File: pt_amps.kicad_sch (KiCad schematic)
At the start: 39 parts, among them J25 Conn_01x04_Female, U11 LM324DT

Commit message: not sure if anything has changed but this is the last commit before moving to two LCs
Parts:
- J25: footprint Connector_PinHeader_2.54mm:PinHeader_1x04_P2.54mm_Vertical -> Connector_PinSocket_2.54mm:PinSocket_1x04_P2.54mm_Vertical
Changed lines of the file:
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@@
       (effects (font (size 1.27 1.27)) (justify left) hide)
     )
-    (property "Footprint" "Connector_PinHeader_2.54mm:PinHeader_1x04_P2.54mm_Vertical" (id 2) (at 127 163.83 0)
+    (property "Footprint" "Connector_PinSocket_2.54mm:PinSocket_1x04_P2.54mm_Vertical" (id 2) (at 127 163.83 0)
       (effects (font (size 1.27 1.27)) hide)
     )

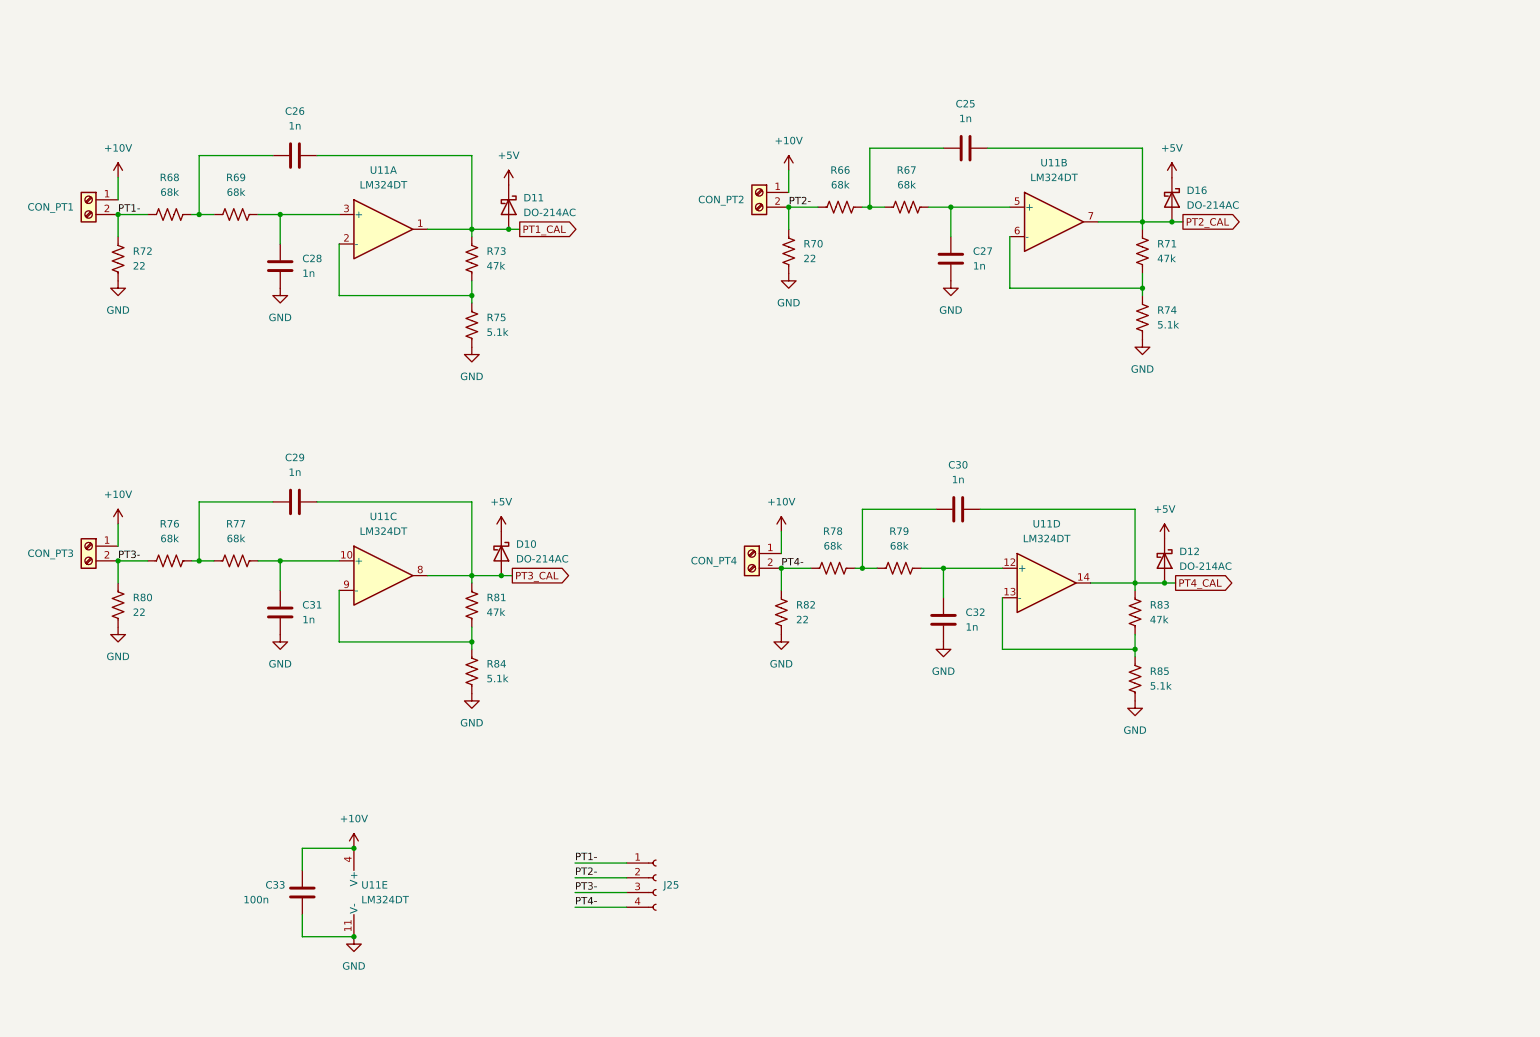
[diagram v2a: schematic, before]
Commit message: done schematiccing after design review
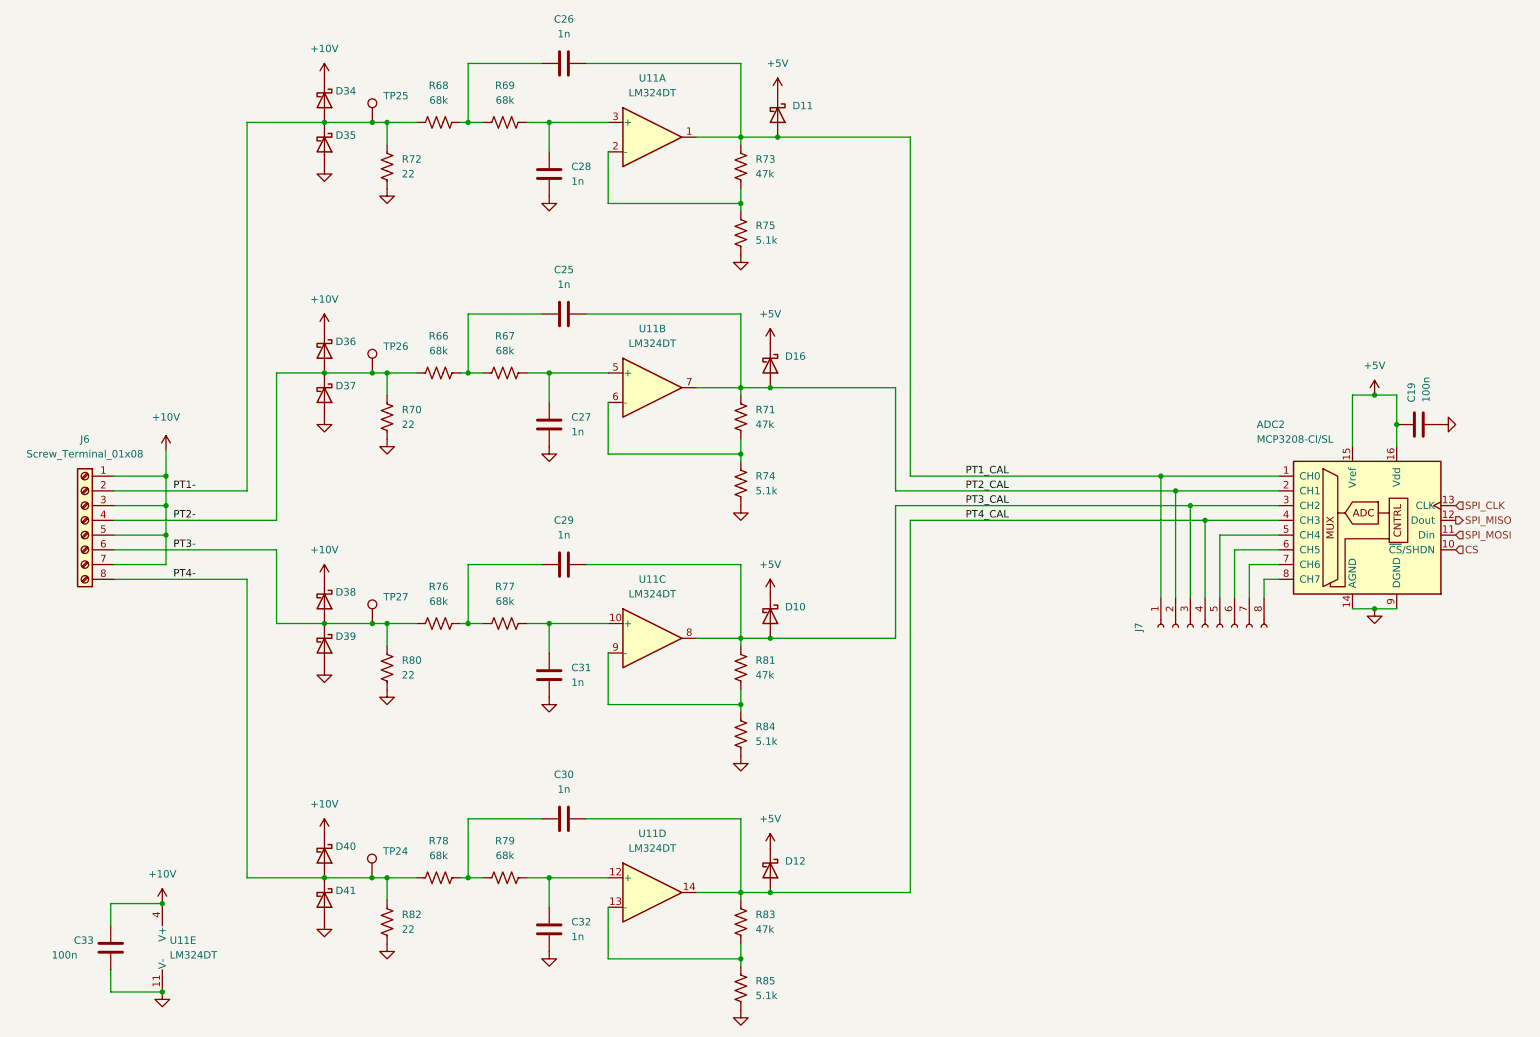
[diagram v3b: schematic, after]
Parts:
- removed CON_PT1, CON_PT2, CON_PT3, CON_PT4: Screw_Terminal_01x02, 1190363:1190363, symbol Connector:Screw_Terminal_01x02
- removed J25: Conn_01x04_Female, Connector_PinSocket_2.54mm:PinSocket_1x04_P2.54mm_Vertical, symbol Connector:Conn_01x04_Female
- added ADC2: MCP3208-CI/SL, Package_SO:SOIC-16_3.9x9.9mm_P1.27mm, symbol Analog_ADC:MCP3208
- added C19: 100n, Capacitor_SMD:C_1206_3216Metric, symbol Device:C
- added D34, D35, D36, D37, D38, D39, D40, D41: CDBA340-HF, Diode_SMD:D_SMA, symbol Device:D_Schottky
- added J6: Screw_Terminal_01x08, symbol Connector:Screw_Terminal_01x08
- added J7: Conn_01x08_Female, Connector_PinSocket_2.54mm:PinSocket_1x08_P2.54mm_Vertical, symbol Connector:Conn_01x08_Female
- added TP24, TP25, TP26, TP27: TestPoint, symbol Connector:TestPoint
- D10, D11, D12, D16: value DO-214AC -> CDBA340-HF; footprint karca_custom_footprints:DO-214AC -> Diode_SMD:D_SMA
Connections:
- net +10V: now also D34.1 (K), D36.1 (K), D38.1 (K), D40.1 (K), J6.1 (Pin_1), J6.3 (Pin_3), J6.5 (Pin_5), J6.7 (Pin_7)
- net +5V: now also ADC2.15 (Vref), ADC2.16 (Vdd), C19.2
- net GND: now also ADC2.14 (AGND), ADC2.9 (DGND), C19.1, D35.2 (A), D37.2 (A), D39.2 (A), D41.2 (A)
- net PT1-: now also D34.2 (A), D35.1 (K), J6.2 (Pin_2), TP25.1
- net PT1_CAL: now also ADC2.1 (CH0), J7.1 (Pin_1)
- net PT2-: now also D36.2 (A), D37.1 (K), J6.4 (Pin_4), TP26.1
- net PT2_CAL: now also ADC2.2 (CH1), J7.2 (Pin_2)
- net PT3-: now also D38.2 (A), D39.1 (K), J6.6 (Pin_6), TP27.1
- net PT3_CAL: now also ADC2.3 (CH2), J7.3 (Pin_3)
- net PT4-: now also D40.2 (A), D41.1 (K), J6.8 (Pin_8), TP24.1
- net PT4_CAL: now also ADC2.4 (CH3), J7.4 (Pin_4)
- new net: ADC2.5 (CH4), J7.5 (Pin_5)
- new net: ADC2.6 (CH5), J7.6 (Pin_6)
- new net: ADC2.7 (CH6), J7.7 (Pin_7)
- new net: ADC2.8 (CH7), J7.8 (Pin_8)
- new net CS: ADC2.10 (~{CS}/SHDN)
- new net SPI_CLK: ADC2.13 (CLK)
- new net SPI_MISO: ADC2.12 (Dout)
- new net SPI_MOSI: ADC2.11 (Din)
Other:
- moved on the sheet: C25, C26, C27, C28, C29, C30, C31, C32, C33, D10, D11, D12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

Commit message: cleaned up PT footprint
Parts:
- J6: footprint (none) -> 1190370:1190370
- TP24, TP25, TP26, TP27: footprint (none) -> TestPoint:TestPoint_Pad_D2.0mm
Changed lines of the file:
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@@
     (property "Reference" "J6" (id 0) (at 28.575 88.265 0))
     (property "Value" "Screw_Terminal_01x08" (id 1) (at 28.575 90.805 0))
-    (property "Footprint" "" (id 2) (at 28.575 102.235 0)
+    (property "Footprint" "1190370:1190370" (id 2) (at 28.575 102.235 0)
       (effects (font (size 1.27 1.27)) hide)
     )
@@
       (effects (font (size 1.27 1.27)) (justify left) hide)
     )
-    (property "Footprint" "" (id 2) (at 83.185 76.835 0)
+    (property "Footprint" "TestPoint:TestPoint_Pad_D2.0mm" (id 2) (at 83.185 76.835 0)
       (effects (font (size 1.27 1.27)) hide)
     )
@@
       (effects (font (size 1.27 1.27)) (justify left) hide)
     )
-    (property "Footprint" "" (id 2) (at 83.1205 163.83 0)
+    (property "Footprint" "TestPoint:TestPoint_Pad_D2.0mm" (id 2) (at 83.1205 163.83 0)
       (effects (font (size 1.27 1.27)) hide)
     )
@@
       (effects (font (size 1.27 1.27)) (justify left) hide)
     )
-    (property "Footprint" "" (id 2) (at 83.185 120.015 0)
+    (property "Footprint" "TestPoint:TestPoint_Pad_D2.0mm" (id 2) (at 83.185 120.015 0)
       (effects (font (size 1.27 1.27)) hide)
     )
@@
       (effects (font (size 1.27 1.27)) (justify left) hide)
     )
-    (property "Footprint" "" (id 2) (at 83.185 33.655 0)
-      (effects (font (size 1.27 1.27)) hide)
-    )
+    (property "Footprint" "TestPoint:TestPoint_Pad_D2.0mm" (id 2) (at 83.185 33.655 0)
+      (effects (font (size 1.27 1.27)) hide)
+    )
